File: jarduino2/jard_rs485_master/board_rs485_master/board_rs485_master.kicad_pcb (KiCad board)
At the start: 2 copper layers, 99 x 69 mm, 2 parts

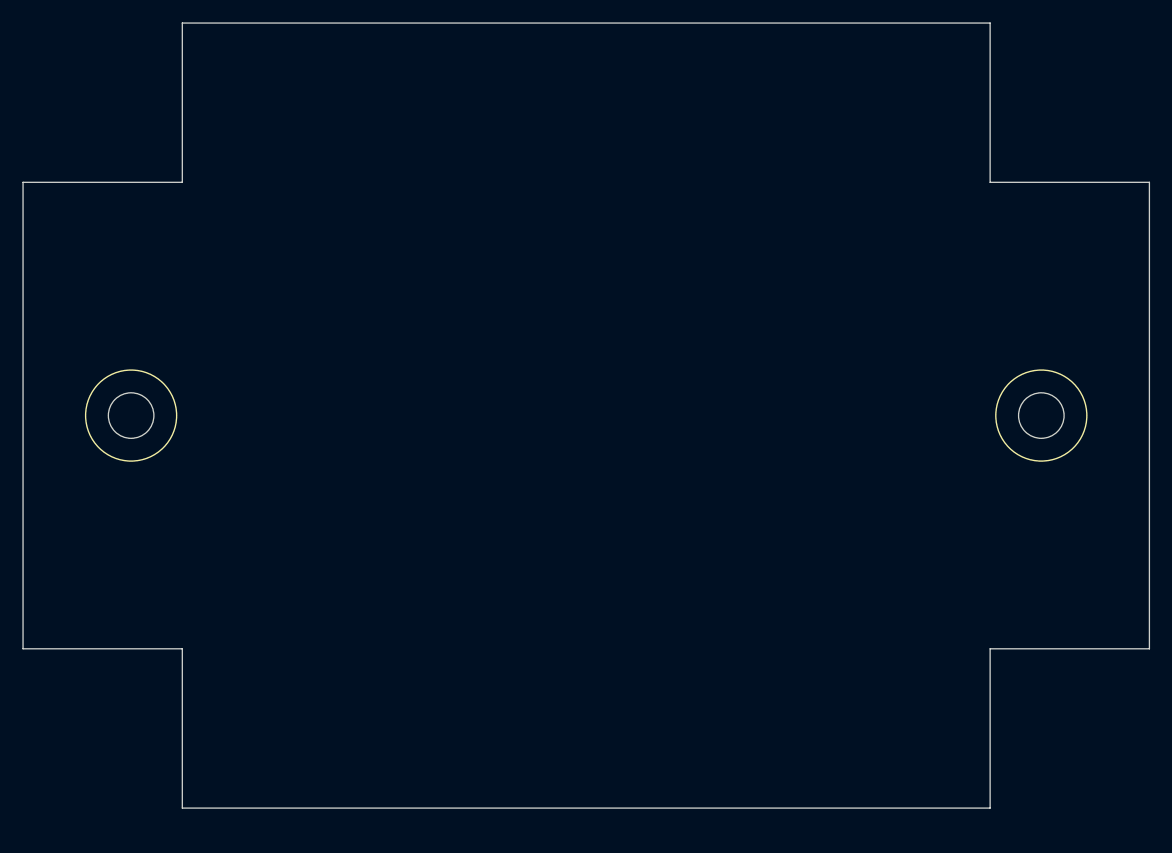
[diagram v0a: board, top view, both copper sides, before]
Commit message: Première visu placement future carte
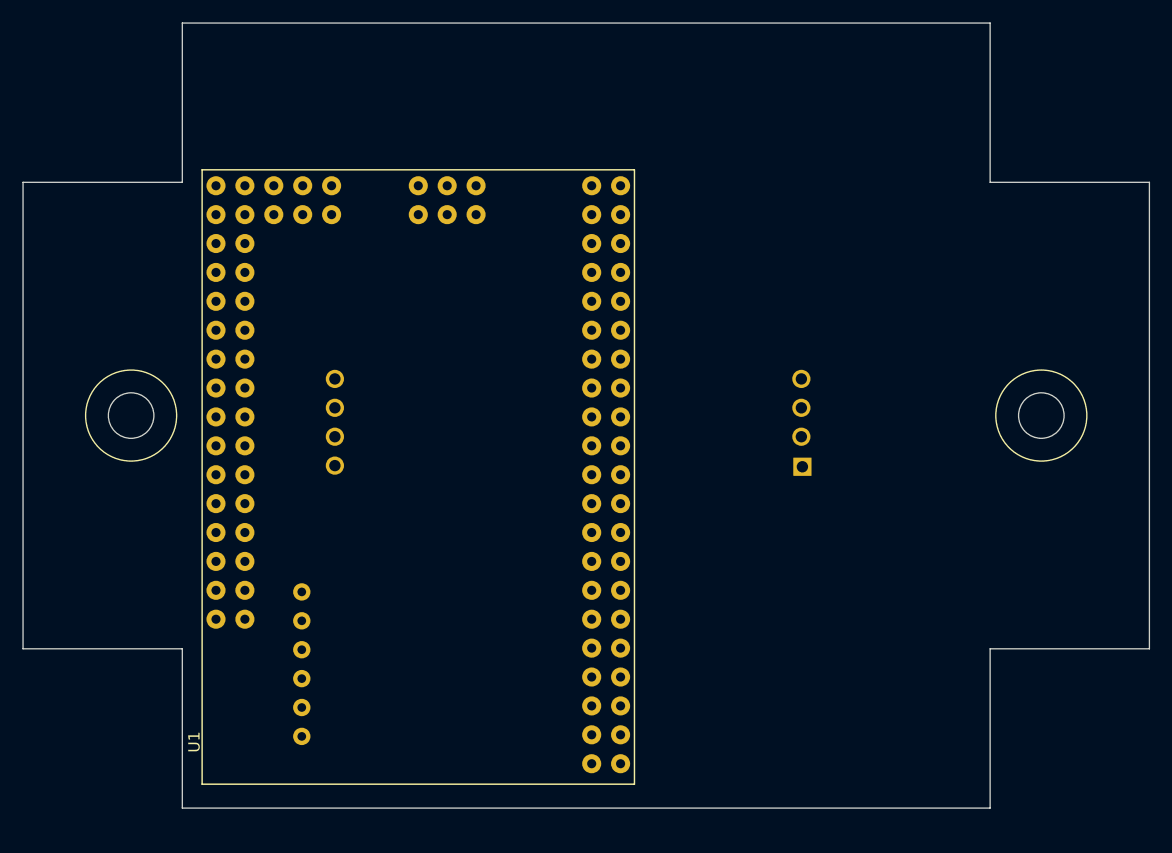
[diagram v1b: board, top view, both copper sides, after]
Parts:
- added U1: MEGA_PRO_EMBED_CH340G_/_ATMEGA2560, bpc:BPC_ATMEGA2560_PRO, F.Cu at (132.7, 103.9)
- added U2: RtcArduino, bpc:BPC_RtcArduino, B.Cu at (122.5, 126.7)
- added U3: Arduino_Mod_RS485, bpc:BPC_Mod485, B.Cu at (166.4, 102.9)
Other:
- net class Default removed

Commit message: Création maître des oyas
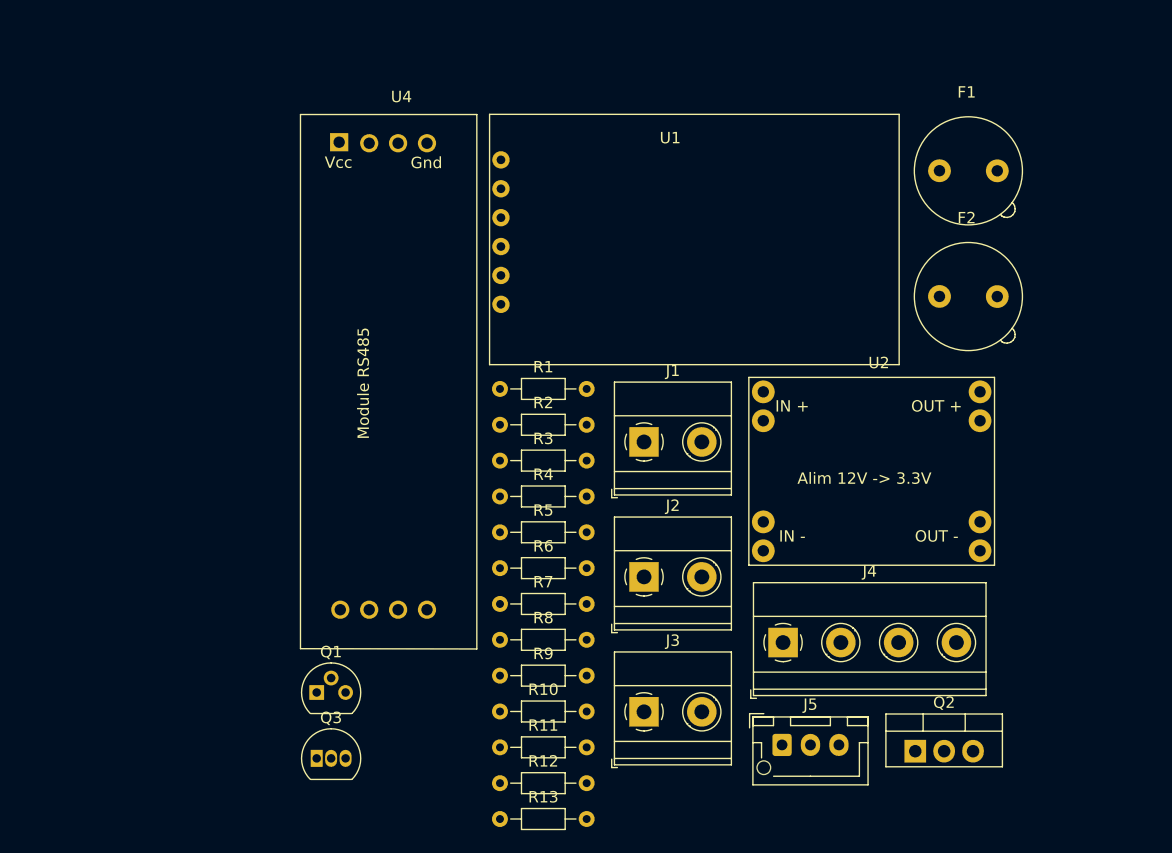
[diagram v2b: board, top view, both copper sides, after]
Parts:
- removed REF** (x2): BPC_Trou4mm_Fixation, bpc:BPC_Trou4mm_Fixation
- removed U3: Arduino_Mod_RS485, bpc:BPC_Mod485
- added F1: Fuse, Fuse:Fuseholder_TR5_Littelfuse_No560_No460, F.Cu at (178.6, 77.0)
- added F2: Fuse, Fuse:Fuseholder_TR5_Littelfuse_No560_No460, F.Cu at (178.6, 88.0)
- added J1: POWER_12V, TerminalBlock_Phoenix:TerminalBlock_Phoenix_MKDS-1,5-2-5.08_1x02_P5.08mm_Horizontal, F.Cu at (152.6, 100.8)
- added J2: ON_OFF, TerminalBlock_Phoenix:TerminalBlock_Phoenix_MKDS-1,5-2-5.08_1x02_P5.08mm_Horizontal, F.Cu at (152.6, 112.7)
- added J3: POWER_OYAS_12V, TerminalBlock_Phoenix:TerminalBlock_Phoenix_MKDS-1,5-2-5.08_1x02_P5.08mm_Horizontal, F.Cu at (152.6, 124.5)
- added J4: BUS_OYAS, TerminalBlock_Phoenix:TerminalBlock_Phoenix_MKDS-1,5-4-5.08_1x04_P5.08mm_Horizontal, F.Cu at (164.8, 118.5)
- added J5: Leds RGB, Connector_JST:JST_XH_B3B-XH-AM_1x03_P2.50mm_Vertical, F.Cu at (164.7, 127.5)
- added Q1: BPC_2N2222A, Package_TO_SOT_THT:TO-92, F.Cu at (123.8, 122.8)
- added Q2: BPC_IPP034N03L, Package_TO_SOT_THT:TO-220-3_Vertical, F.Cu at (176.4, 128.0)
- added Q3: BC327, Package_TO_SOT_THT:TO-92_Inline, F.Cu at (123.8, 128.6)
- added R1: 10k, Resistor_THT:R_Axial_DIN0204_L3.6mm_D1.6mm_P7.62mm_Horizontal, F.Cu at (139.9, 96.2)
- added R10: R, Resistor_THT:R_Axial_DIN0204_L3.6mm_D1.6mm_P7.62mm_Horizontal, F.Cu at (139.9, 124.5)
- added R11: R, Resistor_THT:R_Axial_DIN0204_L3.6mm_D1.6mm_P7.62mm_Horizontal, F.Cu at (139.9, 127.7)
- added R12: R, Resistor_THT:R_Axial_DIN0204_L3.6mm_D1.6mm_P7.62mm_Horizontal, F.Cu at (139.9, 130.8)
- added R13: R, Resistor_THT:R_Axial_DIN0204_L3.6mm_D1.6mm_P7.62mm_Horizontal, F.Cu at (139.9, 134.0)
- added R2: 10k, Resistor_THT:R_Axial_DIN0204_L3.6mm_D1.6mm_P7.62mm_Horizontal, F.Cu at (139.9, 99.3)
- added R3: R, Resistor_THT:R_Axial_DIN0204_L3.6mm_D1.6mm_P7.62mm_Horizontal, F.Cu at (139.9, 102.5)
- added R4: R, Resistor_THT:R_Axial_DIN0204_L3.6mm_D1.6mm_P7.62mm_Horizontal, F.Cu at (139.9, 105.6)
- added R5: R, Resistor_THT:R_Axial_DIN0204_L3.6mm_D1.6mm_P7.62mm_Horizontal, F.Cu at (139.9, 108.8)
- added R6: R, Resistor_THT:R_Axial_DIN0204_L3.6mm_D1.6mm_P7.62mm_Horizontal, F.Cu at (139.9, 111.9)
- added R7: R, Resistor_THT:R_Axial_DIN0204_L3.6mm_D1.6mm_P7.62mm_Horizontal, F.Cu at (139.9, 115.1)
- added R8: R, Resistor_THT:R_Axial_DIN0204_L3.6mm_D1.6mm_P7.62mm_Horizontal, F.Cu at (139.9, 118.2)
- added R9: R, Resistor_THT:R_Axial_DIN0204_L3.6mm_D1.6mm_P7.62mm_Horizontal, F.Cu at (139.9, 121.4)
- added U4: BPC_Mod485, bpc:BPC_Mod485, F.Cu at (125.9, 74.6)
- U1: value MEGA_PRO_EMBED_CH340G_/_ATMEGA2560 -> RtcArduino; footprint bpc:BPC_ATMEGA2560_PRO -> bpc:BPC_RtcArduino
- U2: value RtcArduino -> BPC_Alim3_3V; footprint bpc:BPC_RtcArduino -> bpc:BPC_Alim3_3V; moved to F.Cu
- moved U2 50.6 mm to (163.1, 96.4)
- moved U1 28.8 mm to (140.0, 76.0), turned to 0 degrees
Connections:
- U2 pad 1: unconnected-(U2-GND-Pad1) -> Net-(F1-Pad1)
- U2 pad 2: unconnected-(U2-VCC-Pad2) -> Net-(F1-Pad1)
- U2 pad 3: unconnected-(U2-SDA-Pad3) -> GND
- U2 pad 4: unconnected-(U2-SCL-Pad4) -> GND
- U2 pad 5: unconnected-(U2-SQW-Pad5) -> GND
- U2 pad 6: unconnected-(U2-32K-Pad6) -> GND
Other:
- board outline removed
